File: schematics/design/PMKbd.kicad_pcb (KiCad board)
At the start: 2 copper layers, 28.1 x 39.6 mm, 92 parts, among them J1 Conn_01x01, J10 Conn_01x01, J11 Conn_01x01, J12 Conn_01x01, J13 Conn_01x01, J14 Conn_01x01, J15 Conn_01x01, J16 Conn_01x01, J17 Conn_01x01, J18 Conn_01x01, J19 Conn_01x01, J2 Conn_01x01, J20 Conn_01x01, J21 Conn_01x01, J22 Conn_01x01, J23 Conn_01x01, J24 Conn_01x01, J25 Conn_01x01, J26 Conn_01x01, J27 Conn_01x01, J28 Conn_01x01, J29 Conn_01x01, J3 Conn_01x01, J30 Conn_01x01, J31 Conn_01x01, J32 Conn_01x01, J33 Conn_01x01, J34 Conn_01x01, J35 Conn_01x01, J36 Conn_01x01, J37 Conn_01x01, J38 Conn_01x01, J39 Conn_01x01, J4 Conn_01x01, J40 Conn_01x01, J41 Conn_01x01, J42 Conn_01x01, J43 Conn_01x01, J44 Conn_01x01, J45 Conn_01x01, J46 Conn_01x01, J47 Conn_01x01, J48 Conn_01x01, J49 Conn_01x01, J5 Conn_01x01, J50 Conn_01x01, J51 Conn_01x01, J52 Conn_01x01, J53 Conn_01x01, J54 Conn_01x01, J55 Conn_01x01, J56 Conn_01x01, J57 Conn_01x01, J58 Conn_01x01, J59 Conn_01x01, J6 Conn_01x01, J60 Conn_01x01, J61 Conn_01x01, J62 Conn_01x01, J63 Conn_01x01, J64 Conn_01x01, J65 Conn_01x01, J66 Conn_01x01, J67 Conn_01x01, J68 Conn_01x01, J69 Conn_01x01, J7 Conn_01x01, J70 Conn_01x01, J71 Conn_01x01, J72 Conn_01x01, J73 Conn_01x01, J74 Conn_01x01, J8 Conn_01x01, J9 Conn_01x01, Q1 2N2222, Q2 2N2222, U1 Core51822_(B), U2 LT1117-3.3, U3 MCP73831-2-OT, U4 Core51822_(B)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

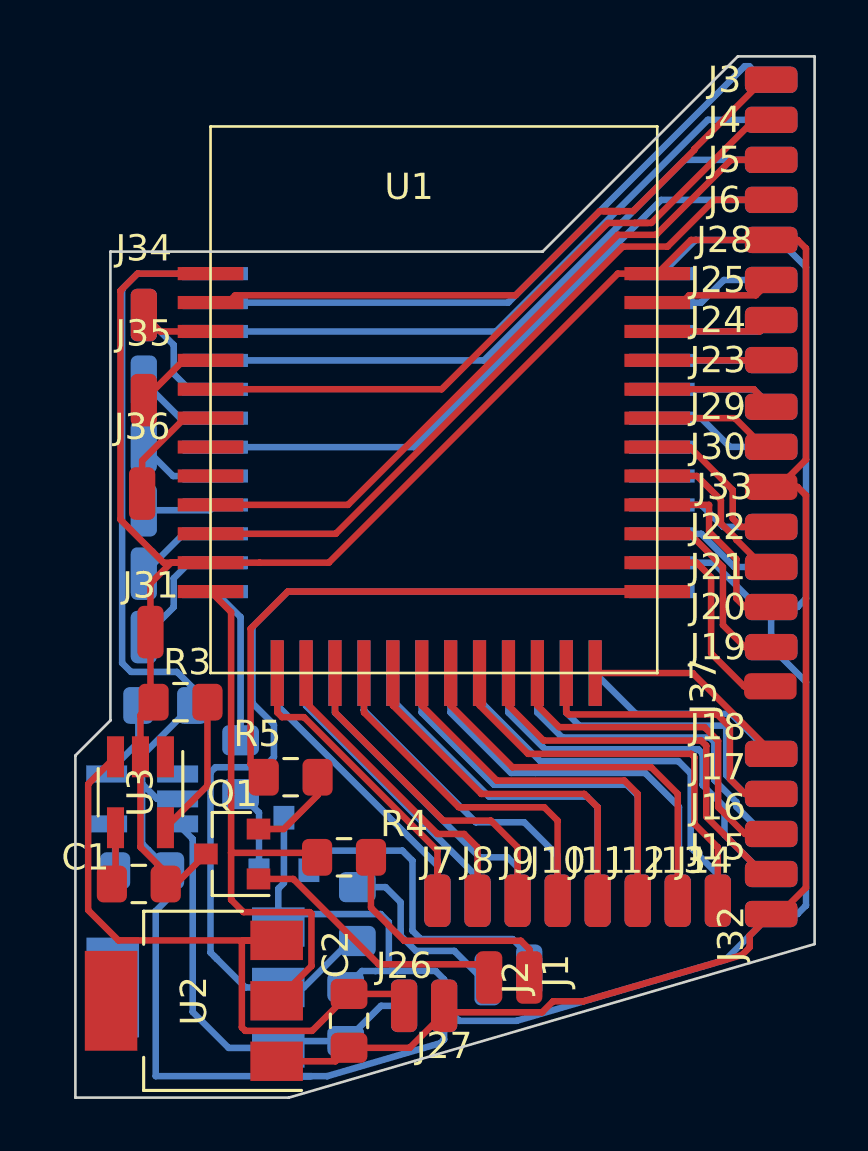
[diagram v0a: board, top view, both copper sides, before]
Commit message: finalized PCB
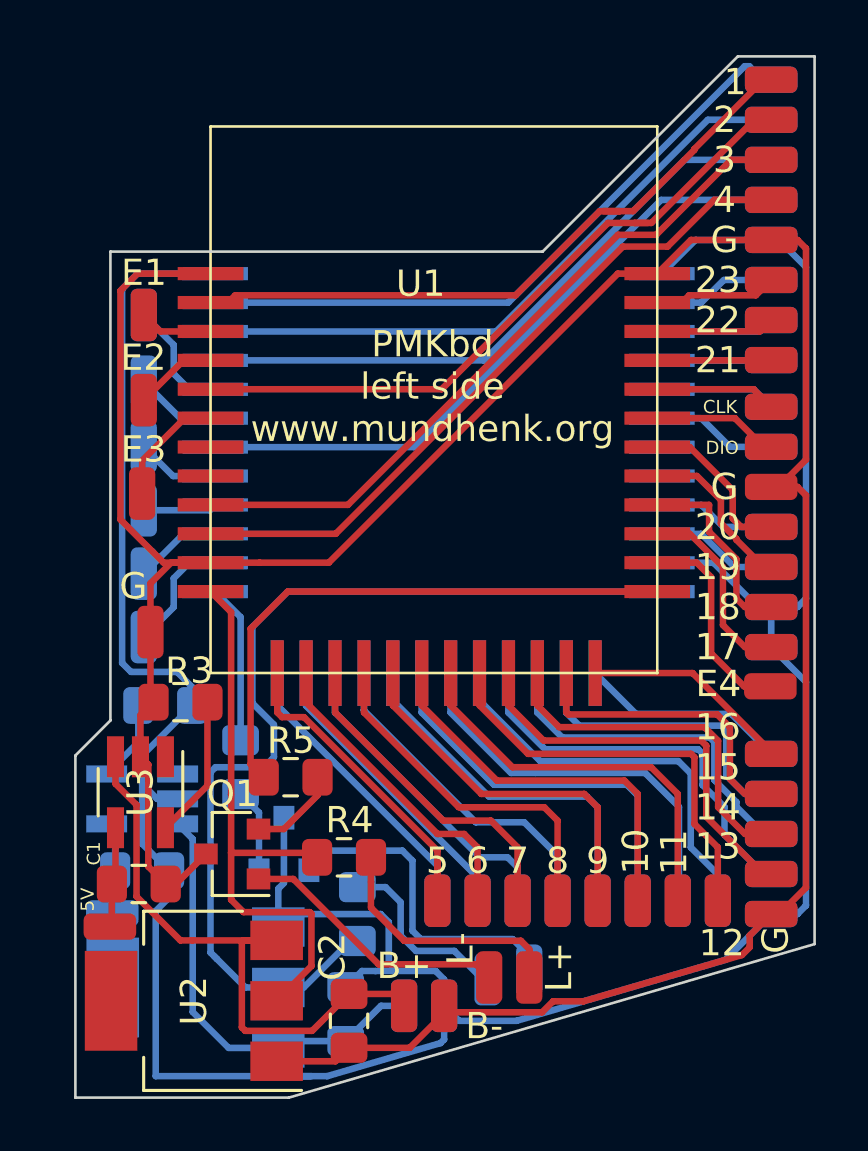
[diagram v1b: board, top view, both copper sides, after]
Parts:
- added 5V: Conn_01x01, Connector_Wire:SolderWirePad_1x01_SMD_1x2mm, B.Cu at (63.3, 95.0)
- added 5V: Conn_01x01, Connector_Wire:SolderWirePad_1x01_SMD_1x2mm, F.Cu at (63.2, 95.5)
- renumbered J3 to 1, J12 to 10, J13 to 11, J14 to 12, J15 to 13, J16 to 14, J17 to 15, J18 to 16, J19 to 17, J20 to 18, J21 to 19, J4 to 2, J22 to 20, J23 to 21, J24 to 22, J25 to 23, J40 to 24, J41 to 25, J42 to 26, J43 to 27, J44 to 28, J45 to 29, J5 to 3, J46 to 30, J47 to 31, J48 to 32, J49 to 33, J50 to 34, J51 to 35, J52 to 36, J53 to 37, J54 to 38, J55 to 39, J6 to 4, J56 to 40, J57 to 41, J58 to 42, J59 to 43, J60 to 44, J61 to 45, J62 to 46, J7 to 5, J8 to 6, J9 to 7, J10 to 8, J11 to 9, J63 to B+, J26 to B+, J27 to B-, J64 to B-, J66 to CLK, J29 to CLK, J67 to DIO, J30 to DIO, J34 to E1, J74 to E1, J35 to E2, J36 to E3, J37 to E4, J71 to E5, J72 to E6, J73 to E7, J69 to G, J70 to G, J68 to G, J65 to G, J32 to G, J33 to G, J31 to G, J28 to G, J1 to L+, J39 to L+, J38 to L-, J2 to L-
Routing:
- net Net-(BT1-Pad1): track 25.5 -> 23.3 mm
- net 5V_R: track 1.92 -> 3.58 mm
- net 5V_L: track 2.20 -> 3.85 mm
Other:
- board text added: "PMKbd left side www.mundhenk.org"
- board text added: "PMKbd right side www.mundhenk.org"
